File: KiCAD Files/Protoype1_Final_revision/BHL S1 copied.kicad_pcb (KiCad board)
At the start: 4 copper layers, 70 x 70 mm, 93 parts, among them IC1 NUP2105LT1G, IC2 NUP2105LT1G, IC4 FD6288Q, J1 39-30-1042, J2 Conn_01x03_Pin, J3 Conn_01x03_Pin, J4 39-30-1042, Q1 CSD19502Q5B, Q2 CSD19502Q5B, Q3 CSD19502Q5B, Q4 CSD19502Q5B, Q5 CSD19502Q5B, Q7 CSD19502Q5B, SW1 PTS636 SM50J SMTR LFS, U1 ME6211C30M5, U2 SPX3819M5-L-5-0, U3 Solder Pad, U5 STM32G431CBU6, Y1 8MHz

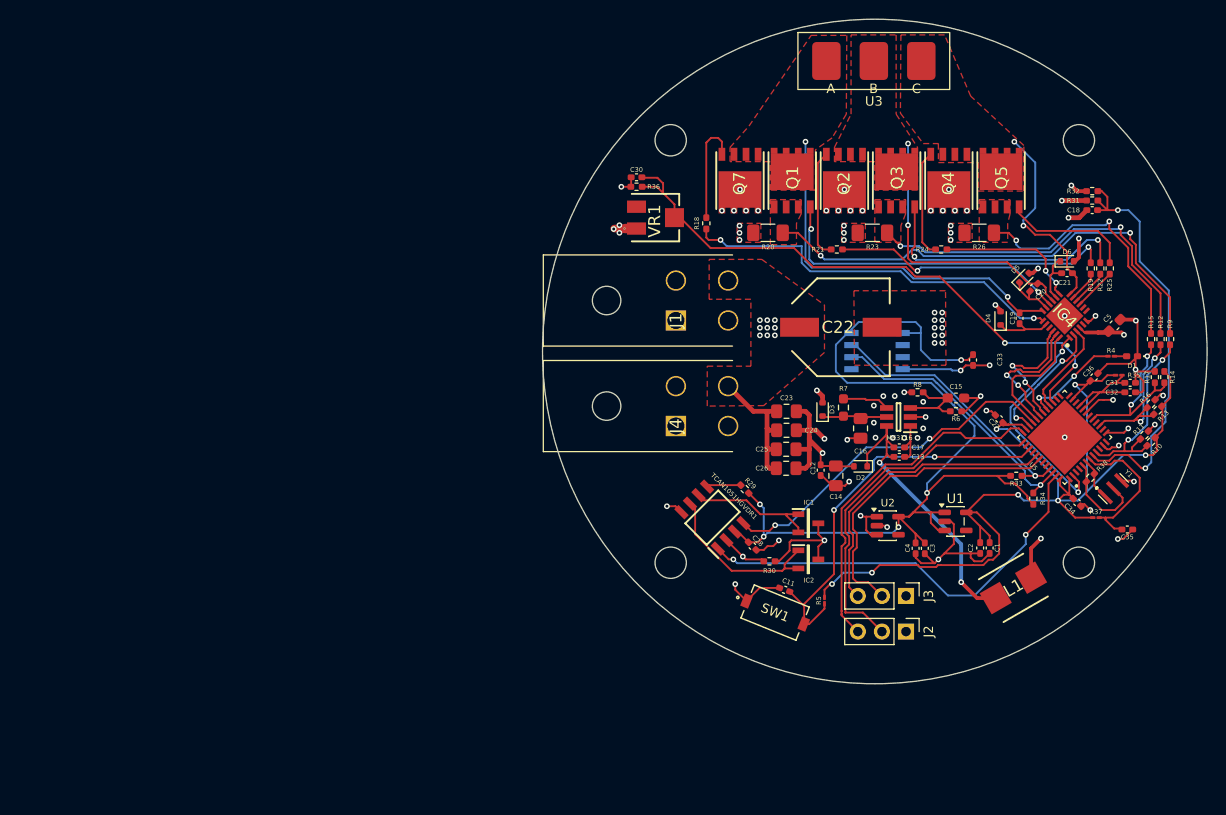
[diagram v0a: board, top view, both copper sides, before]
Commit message: Final Revision of PCB
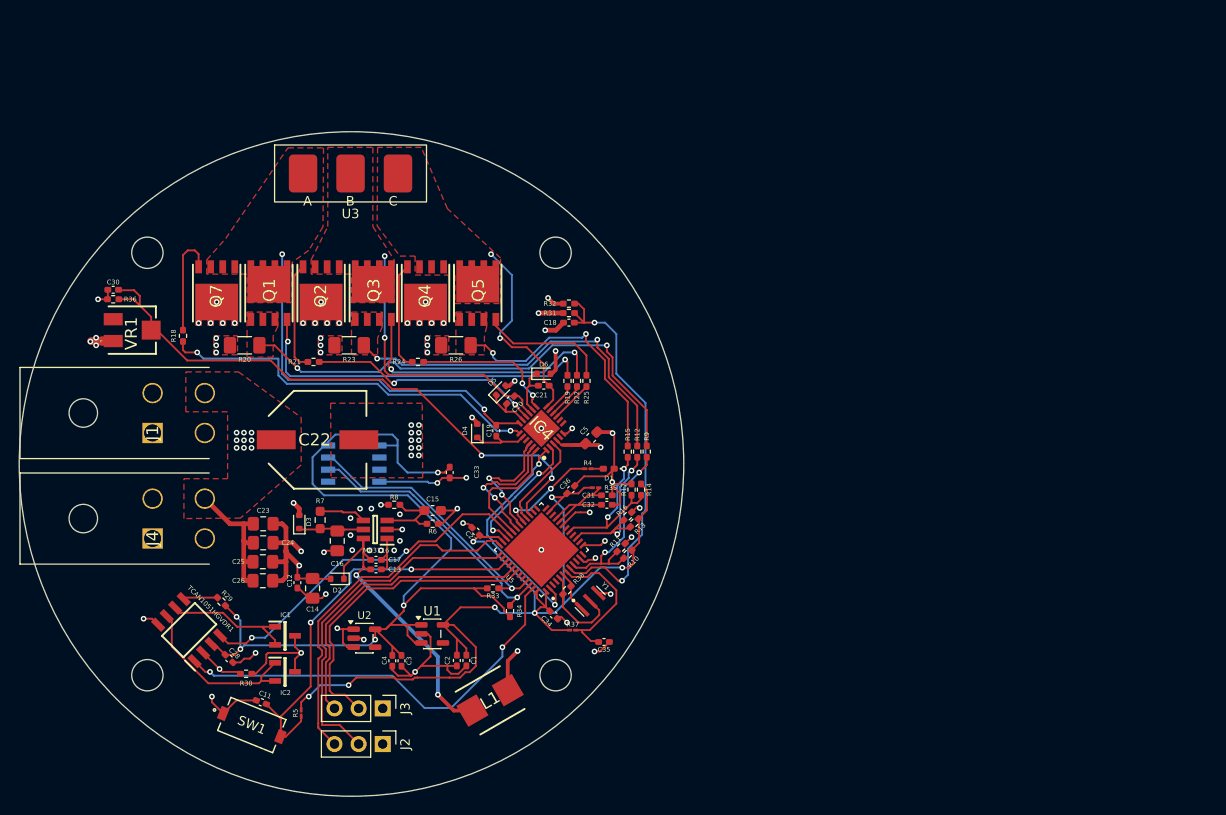
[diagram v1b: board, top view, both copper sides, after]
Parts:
- moved AS5600 56.4 mm to (142.6, 95.3)
- moved C13 56.4 mm to (145.0, 106.5)
- moved C14 56.4 mm to (138.3, 108.5)
- moved C17 56.4 mm to (145.0, 105.5)
- moved C31 56.4 mm to (169.3, 98.7)
- moved C32 56.4 mm to (169.3, 99.7)
- moved J4 56.4 mm to (121.4, 103.2)
- moved R11 56.4 mm to (170.8, 104.2)
- moved R30 56.4 mm to (131.3, 117.5)
- moved R31 56.4 mm to (165.3, 79.5)
- moved R33 56.4 mm to (157.3, 108.5)
- moved R6 56.4 mm to (150.9, 101.7)
- moved U2 56.4 mm to (143.7, 113.7)
- moved U3 56.4 mm to (142.3, 64.8)
- moved C12 56.4 mm to (136.7, 107.8)
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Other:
- outline, holes or cut-outs redrawn
